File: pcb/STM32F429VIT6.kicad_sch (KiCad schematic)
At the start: 22 parts, among them J3 Conn_01x04_Pin, SW1 SW_Push, SW2 SW_Push_SPDT, U2 STM32F429VITx, Y1 Crystal_GND23

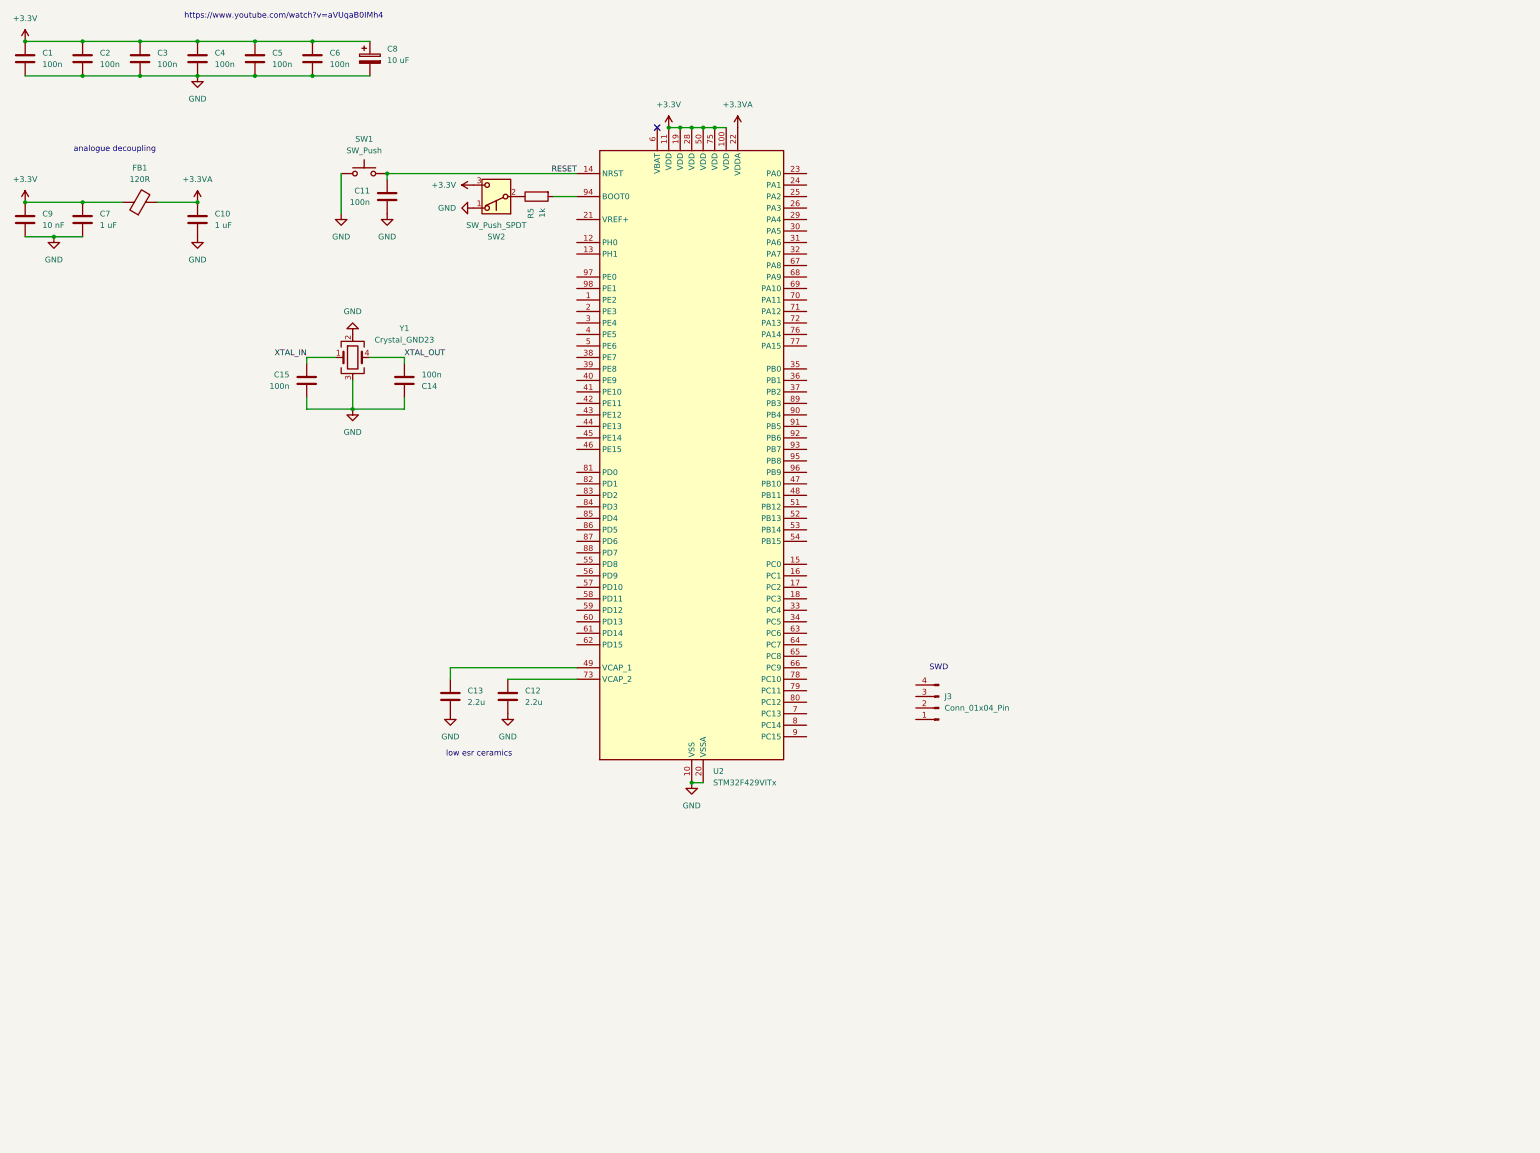
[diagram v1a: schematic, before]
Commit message: 🎛  wip analogue front end
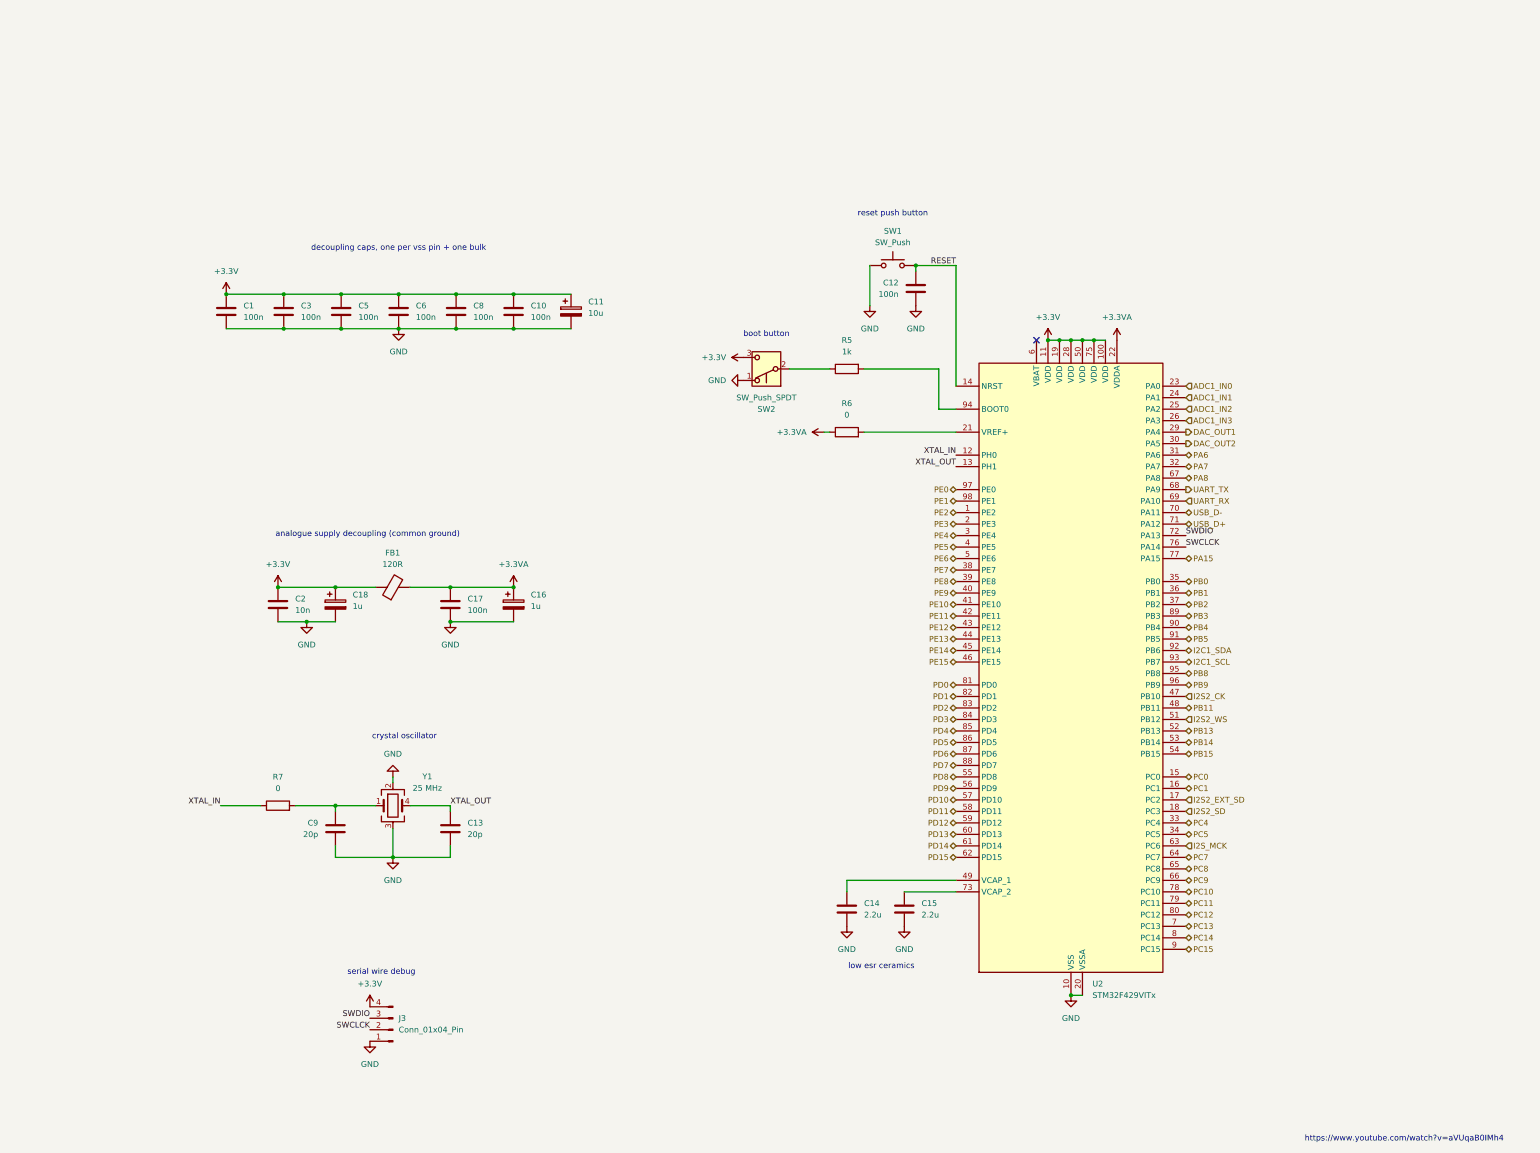
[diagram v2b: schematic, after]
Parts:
- removed C10, C7: 1 uF, Capacitor_SMD:C_0201_0603Metric, symbol Device:C
- added C16, C18: 1u, Capacitor_SMD:CP_Elec_4x3, symbol Device:C_Polarized
- added C17: 100n, Capacitor_SMD:C_0603_1608Metric, symbol Device:C
- added R6, R7: 0, Resistor_SMD:R_0603_1608Metric_Pad0.98x0.95mm_HandSolder, symbol Device:R
- C1: footprint Capacitor_SMD:C_0201_0603Metric -> Capacitor_SMD:C_0603_1608Metric
- C10: renamed from C6; footprint Capacitor_SMD:C_0201_0603Metric -> Capacitor_SMD:C_0603_1608Metric
- C11: renamed from C8; value 10 uF -> 10u
- C12: renamed from C11; footprint Capacitor_SMD:C_0201_0603Metric -> Capacitor_SMD:C_0603_1608Metric
- C13: renamed from C14; value 100n -> 20p; footprint Capacitor_SMD:C_0201_0603Metric -> Capacitor_SMD:C_0603_1608Metric
- C14: renamed from C13; footprint Capacitor_SMD:C_0201_0603Metric -> Capacitor_SMD:C_0603_1608Metric
- C15: renamed from C12; footprint Capacitor_SMD:C_0201_0603Metric -> Capacitor_SMD:C_0603_1608Metric
- C2: renamed from C9; value 10 nF -> 10n; footprint Capacitor_SMD:C_0201_0603Metric -> Capacitor_SMD:C_0603_1608Metric
- C3: renamed from C2; footprint Capacitor_SMD:C_0201_0603Metric -> Capacitor_SMD:C_0603_1608Metric
- C5: renamed from C3; footprint Capacitor_SMD:C_0201_0603Metric -> Capacitor_SMD:C_0603_1608Metric
- C6: renamed from C4; footprint Capacitor_SMD:C_0201_0603Metric -> Capacitor_SMD:C_0603_1608Metric
- C8: renamed from C5; footprint Capacitor_SMD:C_0201_0603Metric -> Capacitor_SMD:C_0603_1608Metric
- C9: renamed from C15; value 100n -> 20p; footprint Capacitor_SMD:C_0201_0603Metric -> Capacitor_SMD:C_0603_1608Metric
- FB1: footprint (none) -> Resistor_SMD:R_0603_1608Metric
- J3: footprint (none) -> Connector_PinHeader_2.54mm:PinHeader_1x04_P2.54mm_Vertical
- R5: footprint (none) -> Resistor_SMD:R_0603_1608Metric_Pad0.98x0.95mm_HandSolder
- SW1: footprint (none) -> Button_Switch_SMD:Panasonic_EVQPUK_EVQPUB
- SW2: footprint (none) -> Button_Switch_SMD:SW_SPDT_PCM12
- Y1: value Crystal_GND23 -> 25 MHz
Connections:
- net +3.3V: now also J3.4 (Pin_4), C18.1
- net +3.3VA: now also C16.1, C17.1, R6.1
- net GND: now also C13.2, J3.1 (Pin_1), C16.2, C17.2, C18.2; no longer C13.1
- net XTAL_IN: now also U2.12 (PH0), R7.1; no longer C9.1, Y1.1
- net XTAL_OUT: now also C13.1, U2.13 (PH1); no longer C13.2
- net PE2: now reaches U2.1 (PE2)
- net PC0: now reaches U2.15 (PC0)
- net PC1: now reaches U2.16 (PC1)
- net I2S2_EXT_SD: now reaches U2.17 (PC2)
- net I2S2_SD: now reaches U2.18 (PC3)
- net PE3: now reaches U2.2 (PE3)
- net at U2.21 (VREF+): now also R6.2
- net ADC1_IN0: now reaches U2.23 (PA0)
- net ADC1_IN1: now reaches U2.24 (PA1)
- net ADC1_IN2: now reaches U2.25 (PA2)
- net ADC1_IN3: now reaches U2.26 (PA3)
- net DAC_OUT1: now reaches U2.29 (PA4)
- net PE4: now reaches U2.3 (PE4)
- net DAC_OUT2: now reaches U2.30 (PA5)
- net PA6: now reaches U2.31 (PA6)
- net PA7: now reaches U2.32 (PA7)
- net PC4: now reaches U2.33 (PC4)
- net PC5: now reaches U2.34 (PC5)
- net PB0: now reaches U2.35 (PB0)
- net PB1: now reaches U2.36 (PB1)
- net PB2: now reaches U2.37 (PB2)
- net PE7: now reaches U2.38 (PE7)
- net PE8: now reaches U2.39 (PE8)
- net PE5: now reaches U2.4 (PE5)
- net PE9: now reaches U2.40 (PE9)
- net PE10: now reaches U2.41 (PE10)
- net PE11: now reaches U2.42 (PE11)
- net PE12: now reaches U2.43 (PE12)
- net PE13: now reaches U2.44 (PE13)
- net PE14: now reaches U2.45 (PE14)
- net PE15: now reaches U2.46 (PE15)
- net I2S2_CK: now reaches U2.47 (PB10)
- net PB11: now reaches U2.48 (PB11)
- net PE6: now reaches U2.5 (PE6)
- net I2S2_WS: now reaches U2.51 (PB12)
- net PB13: now reaches U2.52 (PB13)
- net PB14: now reaches U2.53 (PB14)
- net PB15: now reaches U2.54 (PB15)
- net PD8: now reaches U2.55 (PD8)
- net PD9: now reaches U2.56 (PD9)
- net PD10: now reaches U2.57 (PD10)
- net PD11: now reaches U2.58 (PD11)
- net PD12: now reaches U2.59 (PD12)
- net PD13: now reaches U2.60 (PD13)
- net PD14: now reaches U2.61 (PD14)
- net PD15: now reaches U2.62 (PD15)
- net I2S_MCK: now reaches U2.63 (PC6)
- net PC7: now reaches U2.64 (PC7)
- net PC8: now reaches U2.65 (PC8)
- net PC9: now reaches U2.66 (PC9)
- net PA8: now reaches U2.67 (PA8)
- net UART_TX: now reaches U2.68 (PA9)
- net UART_RX: now reaches U2.69 (PA10)
- net PC13: now reaches U2.7 (PC13)
- net USB_D-: now reaches U2.70 (PA11)
- net USB_D+: now reaches U2.71 (PA12)
- net SWDIO: now reaches U2.72 (PA13)
- net SWDIO: now also J3.3 (Pin_3)
- net SWCLCK: now reaches U2.76 (PA14)
- net SWCLCK: now also J3.2 (Pin_2)
- net PA15: now reaches U2.77 (PA15)
- net PC10: now reaches U2.78 (PC10)
- net PC11: now reaches U2.79 (PC11)
- net PC14: now reaches U2.8 (PC14)
- net PC12: now reaches U2.80 (PC12)
- net PD0: now reaches U2.81 (PD0)
- net PD1: now reaches U2.82 (PD1)
- net PD2: now reaches U2.83 (PD2)
- net PD3: now reaches U2.84 (PD3)
- net PD4: now reaches U2.85 (PD4)
- net PD5: now reaches U2.86 (PD5)
- net PD6: now reaches U2.87 (PD6)
- net PD7: now reaches U2.88 (PD7)
- net PB3: now reaches U2.89 (PB3)
- net PC15: now reaches U2.9 (PC15)
- net PB4: now reaches U2.90 (PB4)
- net PB5: now reaches U2.91 (PB5)
- net I2C1_SDA: now reaches U2.92 (PB6)
- net I2C1_SCL: now reaches U2.93 (PB7)
- net PB8: now reaches U2.95 (PB8)
- net PB9: now reaches U2.96 (PB9)
- net PE0: now reaches U2.97 (PE0)
- net PE1: now reaches U2.98 (PE1)
- new net: C9.1, R7.2, Y1.1
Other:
- note added: "analogue supply decoupling (common ground)"
- note added: "boot button"
- note added: "crystal oscillator"
- note added: "decoupling caps, one per vss pin + one bulk"
- note added: "reset push button"
- note added: "serial wire debug"
- note removed: "SWD"
- note removed: "analogue decoupling"
- company: (none) -> kevontheweb
- title: (none) -> STM32F429VIT6
- moved on the sheet: C1, C10, C11, C12, C13, C14, C15, C2, C3, C5, C6, C8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
